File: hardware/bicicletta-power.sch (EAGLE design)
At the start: 20 parts, among them IC1 LM5017

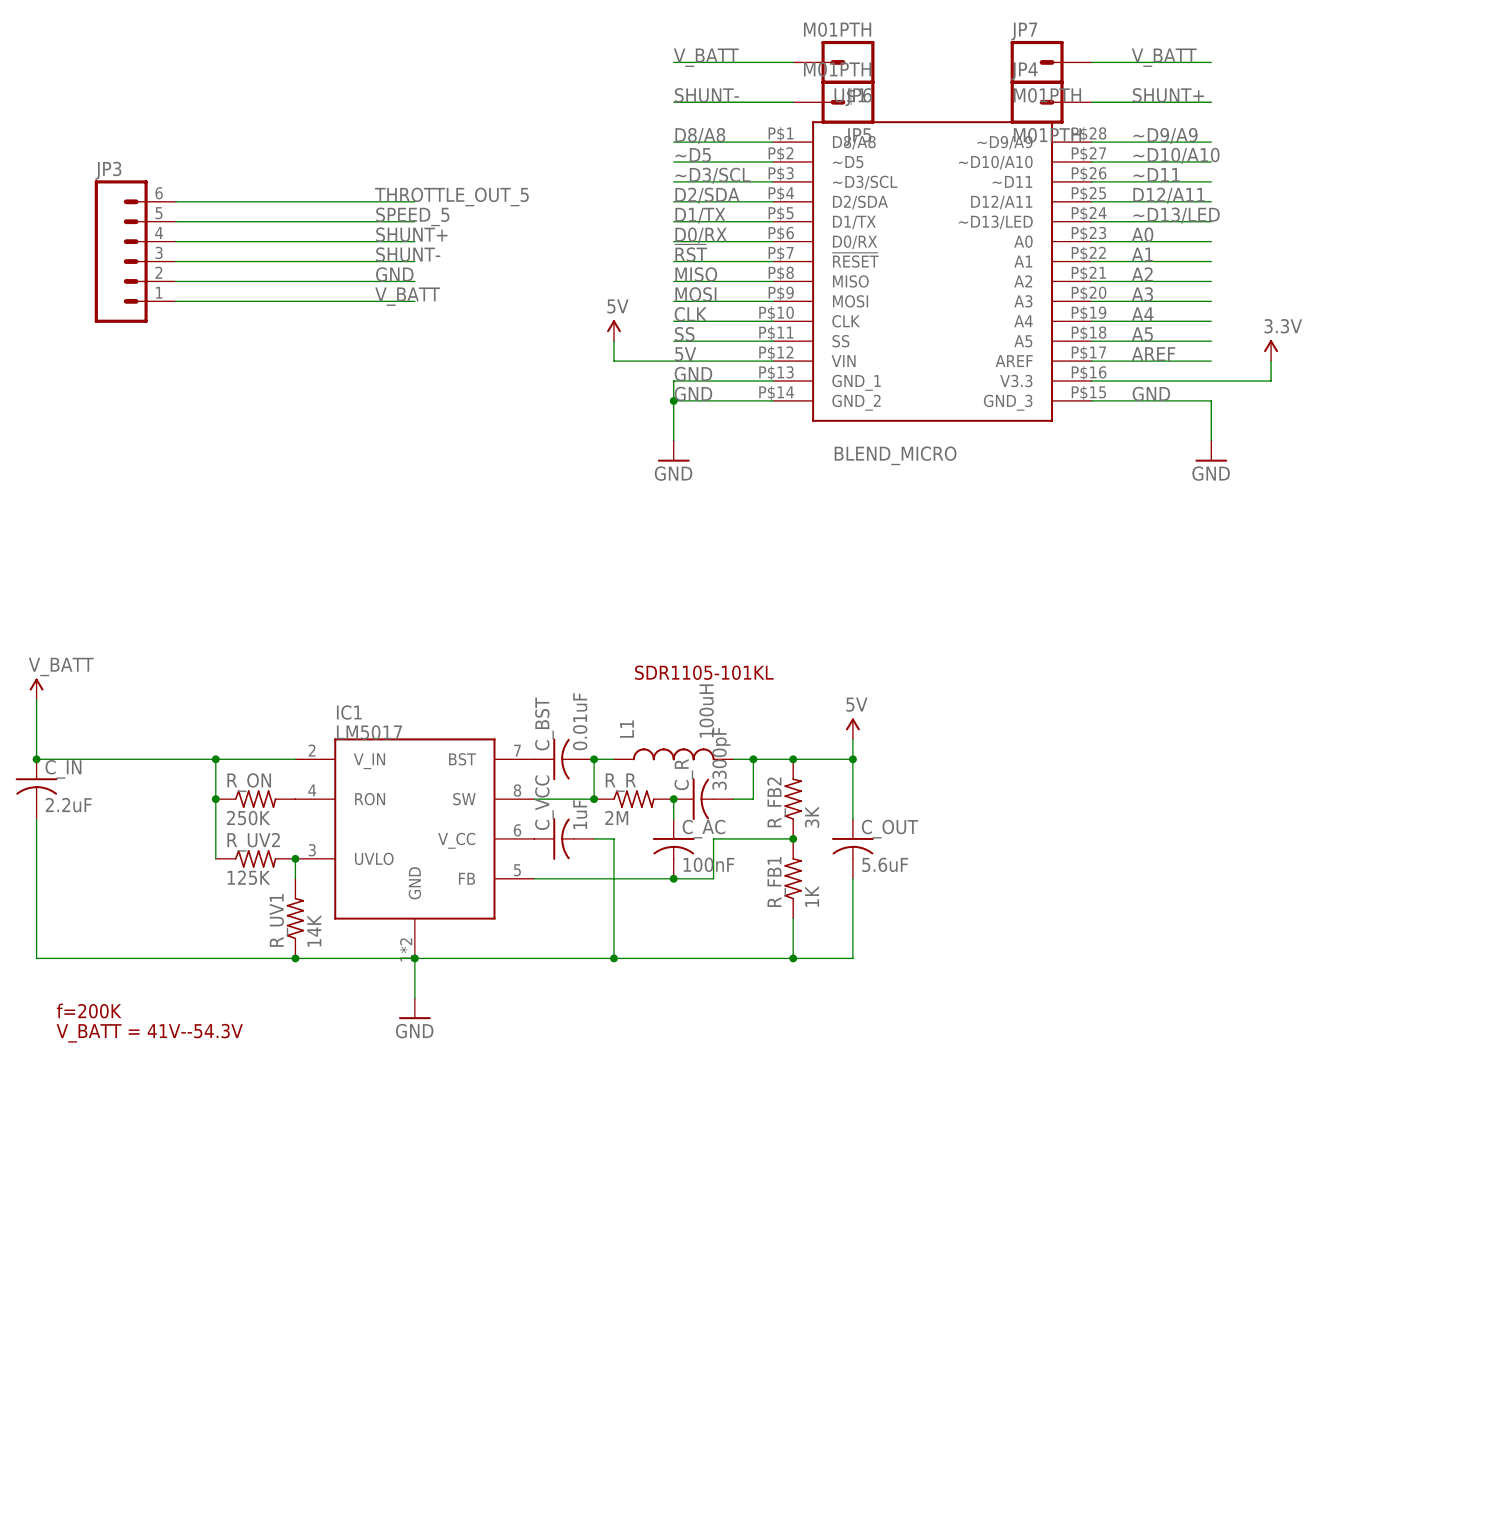
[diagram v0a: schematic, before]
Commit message: There it is. Order that.
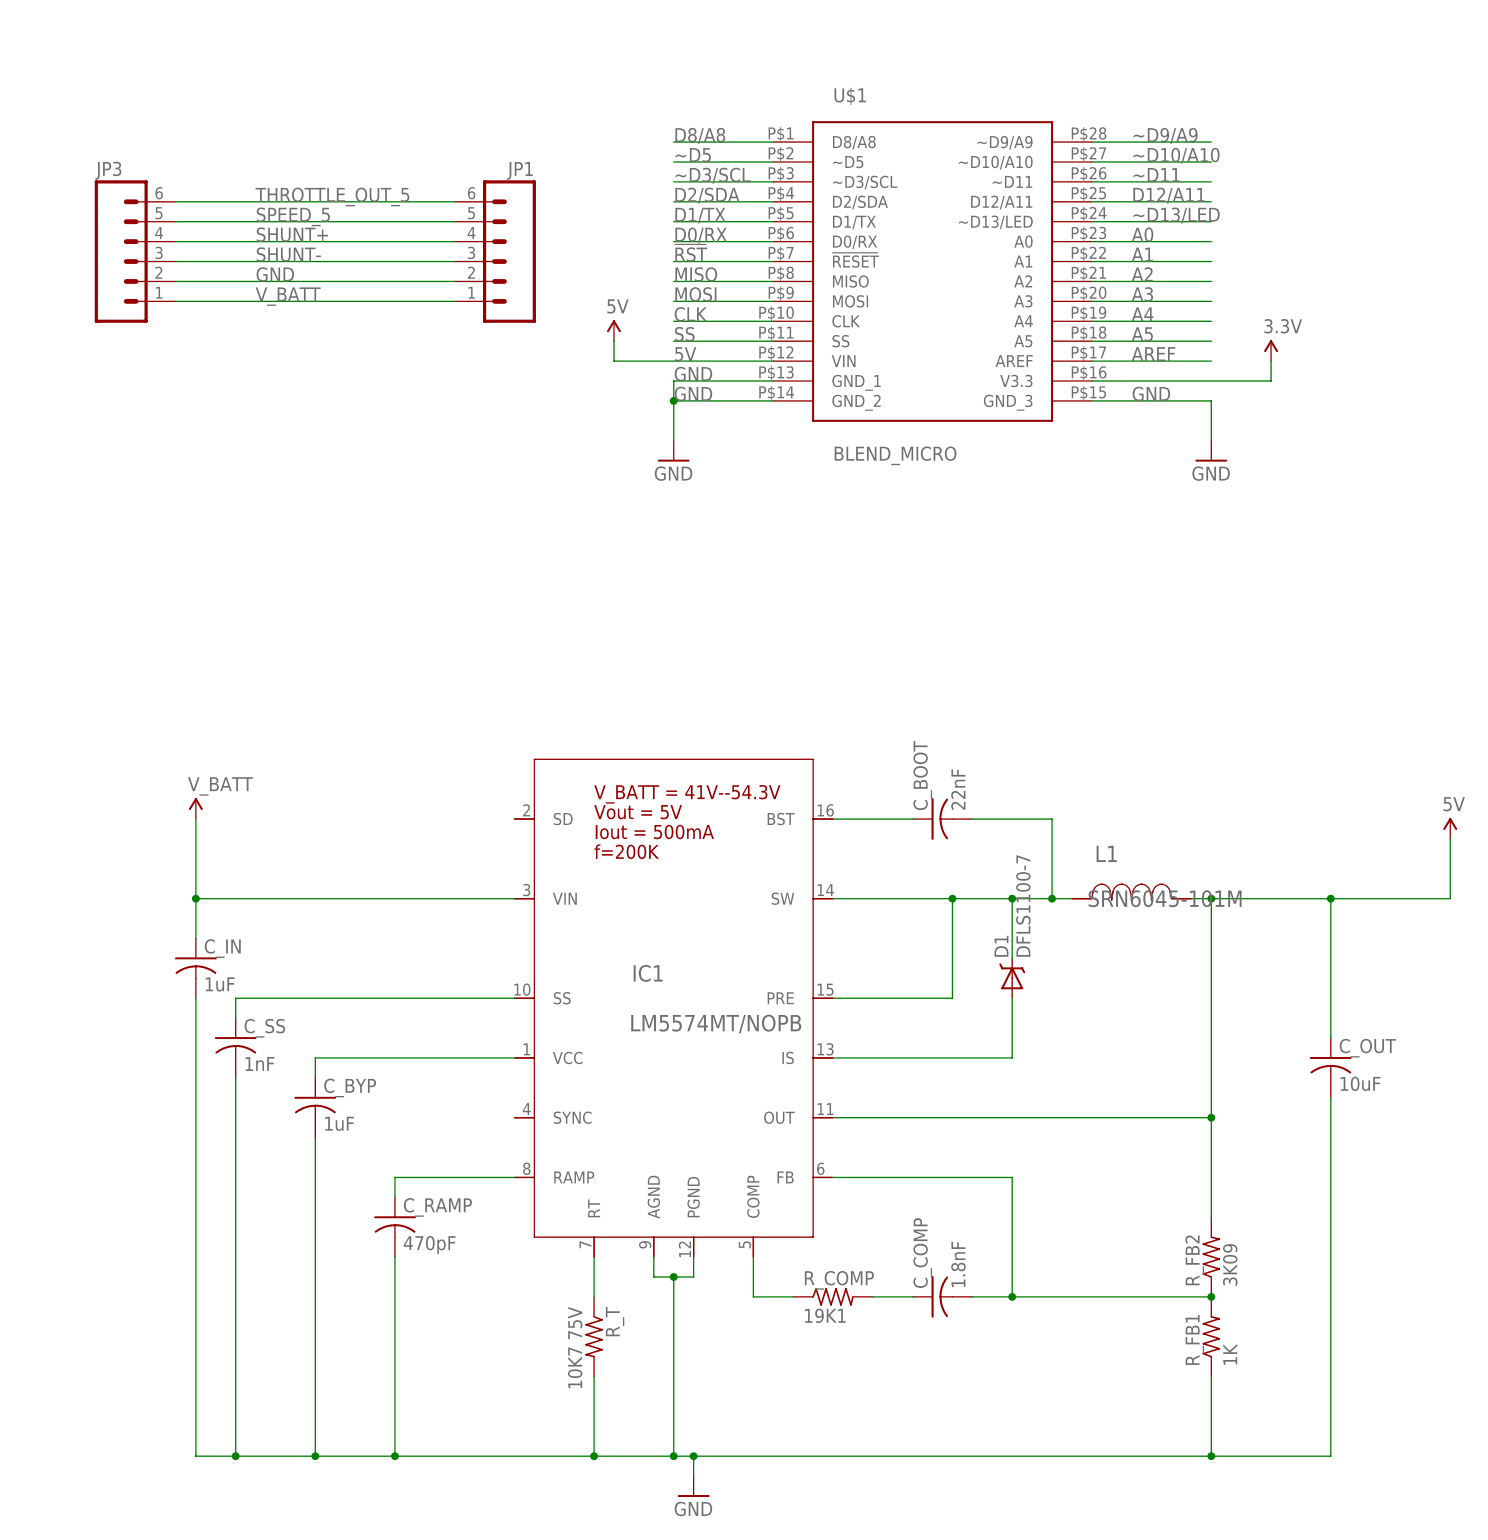
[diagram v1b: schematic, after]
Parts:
- removed C_AC: 100nF, rcl:C-USC0603
- removed C_BST: 0.01uF, rcl:C-USC0603
- removed C_R: 3300pF, rcl:C-USC0603
- removed C_VCC: 1uF, rcl:C-USC0603
- removed JP4, JP5, JP6, JP7: M01PTH, SparkFun-Connectors:M01PTH
- removed R_ON: 250K, rcl:R-US_M0805
- removed R_R: 2M, rcl:R-US_M0805
- removed R_UV1: 14K, rcl:R-US_M0805
- removed R_UV2: 125K, rcl:R-US_M0805
- added C_BOOT: 22nF, rcl:C-USC0603
- added C_BYP: 1uF, rcl:C-USC0603
- added C_COMP: 1.8nF, rcl:C-USC0603
- added C_RAMP: 470pF, rcl:C-USC0603
- added C_SS: 1nF, rcl:C-USC0603
- added D1: DFLS1100-7, TI:DFLS1100-7
- added JP1: (no value), SparkFun-Connectors:M06SIP
- added R_COMP: 19K1, rcl:R-US_R0603
- added R_T: 10K7 75V, rcl:R-US_R0603
- C_IN: value 2.2uF -> 1uF; device rcl:C-USC1210K -> rcl:C-USC1206
- C_OUT: value 5.6uF -> 10uF; device rcl:C-USC0603 -> rcl:C-USC0805
- IC1: value LM5017 -> LM5574MT/NOPB; device Railstars:LM5017 -> TI:LM5574MT/NOPB
- L1: value 100uH -> SRN6045-101M; device Railstars:SRN1060 -> TI:SRN6045-101M
- R_FB1: device rcl:R-US_M0805 -> rcl:R-US_R0603
- R_FB2: value 3K -> 3K09; device rcl:R-US_M0805 -> rcl:R-US_R0603
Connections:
- removed net N$4: C_BST.2, IC1.SW, L1.1, R_R.1
- new net N$10: C_BOOT.1, IC1.BST
- new net N$11: C_BOOT.2, D1.K, IC1.PRE, IC1.SW, L1.1
- new net N$5: IC1.RT, R_T.1
- new net N$8: IC1.COMP, R_COMP.1
- net 5V: now also IC1.OUT; no longer C_R.2
- net GND: now also C_BYP.2, C_RAMP.2, C_SS.2, IC1.AGND, IC1.PGND, JP1.2, R_T.2; no longer C_VCC.2, IC1.GND, R_UV1.1
- net N$1: now also C_SS.1, IC1.SS; no longer IC1.RON, R_ON.2
- net N$2: now also C_BYP.1, IC1.VCC; no longer C_AC.2, IC1.FB, R_FB1.2, R_FB2.1
- net N$3: now also C_RAMP.1, IC1.RAMP; no longer IC1.UVLO, R_UV1.2, R_UV2.2
- net N$6: now also C_COMP.2, IC1.FB, R_FB1.2, R_FB2.1; no longer C_AC.1, C_R.1, R_R.2
- net N$7: now also C_COMP.1, R_COMP.2; no longer C_BST.1, IC1.BST
- net N$9: now also D1.A, IC1.IS; no longer C_VCC.1, IC1.V_CC
- net SHUNT+: now also JP1.4; no longer JP4.1
- net SHUNT-: now also JP1.3; no longer JP5.1
- net SPEED_5: now also JP1.5
- net THROTTLE_OUT_5: now also JP1.6
- net V_BATT: now also IC1.VIN, JP1.1; no longer IC1.V_IN, JP6.1, JP7.1, R_ON.1, R_UV2.1
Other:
- note added: "Iout = 500mA"
- note added: "Vout = 5V"
- note removed: "SDR1105-101KL"
- moved on the sheet: C_IN, C_OUT, R_FB1, R_FB2
